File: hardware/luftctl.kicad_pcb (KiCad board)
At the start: 2 copper layers, 84 x 53.5 mm, 40 parts, among them J1 USB_C_Receptacle_USB2.0, J2 UART, J3 I2C, J4 PWM Fan, J5 PWM Fan, SW1 Reset, U1 LMR62014XMF, U2 MIC5504-3.3YM5, U3 USBLC6-4SC6, U4 ESP32-C3-WROOM-02

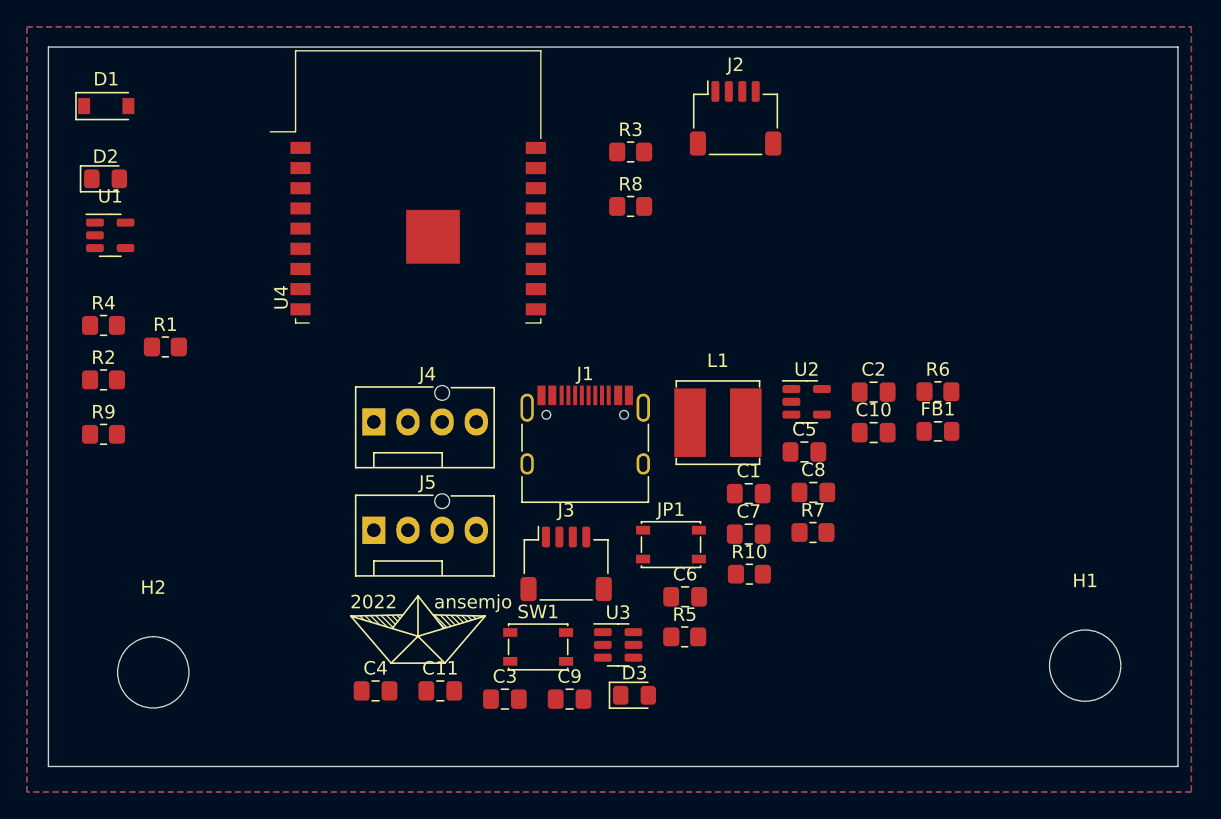
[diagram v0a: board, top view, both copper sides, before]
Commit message: finished pcb layout
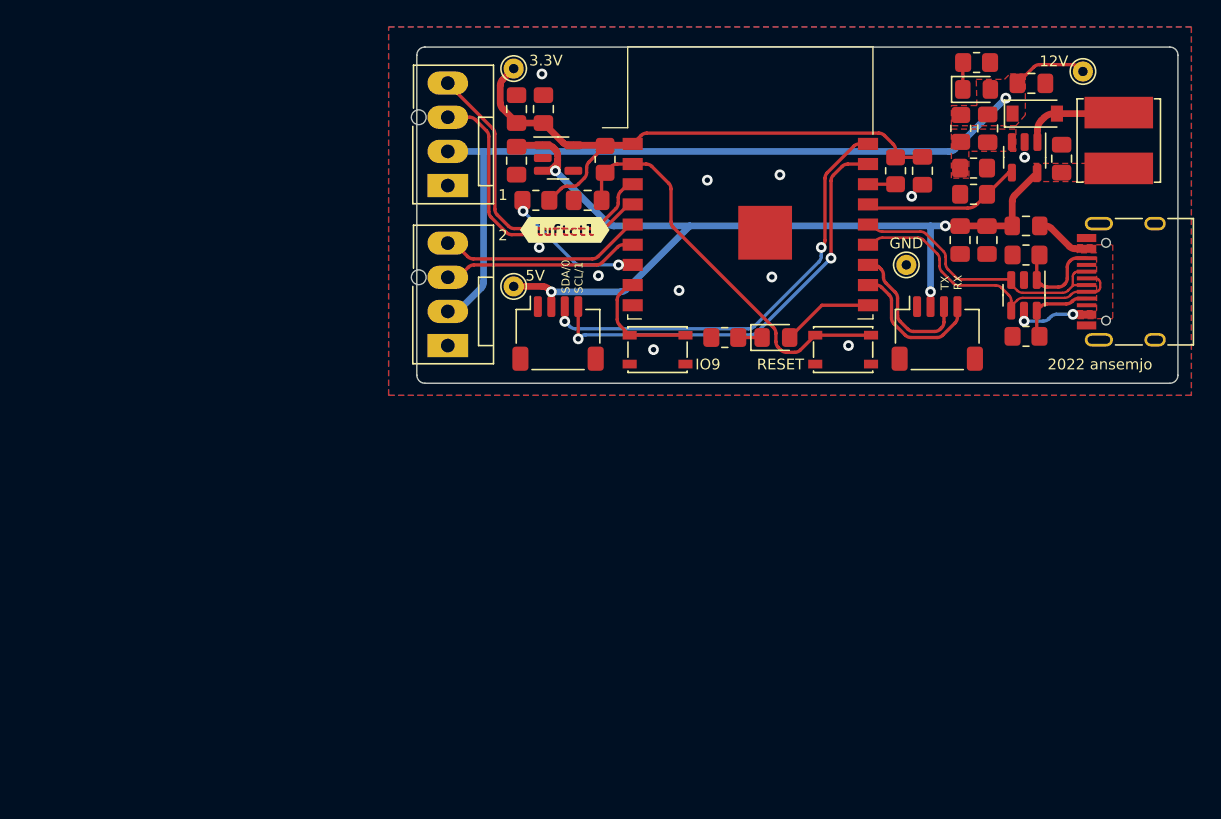
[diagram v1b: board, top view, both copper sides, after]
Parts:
- removed A1: 2022, ansemjo:ahoi
- removed C2: DNP, Capacitor_SMD:C_0805_2012Metric_Pad1.18x1.45mm_HandSolder
- removed H1, H2: MountingHole, MountingHole:MountingHole_5.3mm_M5
- added TP1: Test, TestPoint:TestPoint_THTPad_D1.5mm_Drill0.7mm, F.Cu at (175.1, 51.8)
- added TP2: Test, TestPoint:TestPoint_THTPad_D1.5mm_Drill0.7mm, F.Cu at (132.8, 67.8)
- added TP3: Test, TestPoint:TestPoint_THTPad_D1.5mm_Drill0.7mm, F.Cu at (132.8, 51.6)
- added TP4: Test, TestPoint:TestPoint_THTPad_D1.5mm_Drill0.7mm, F.Cu at (162.0, 66.2)
- added kibuzzard-61E47F36: G***, kibuzzard-61E47F36, F.Cu at (136.6, 63.6)
- moved D1 69.1 mm to (171.6, 55.0)
- moved R4 68.6 mm to (170.9, 71.5), turned to 180 degrees
- moved U1 68.2 mm to (170.8, 58.2), turned to -90 degrees
- moved R2 66.6 mm to (167.0, 59.0)
- moved R1 61.3 mm to (166.1, 56.0), turned to -90 degrees
- moved D3 51.7 mm to (167.2, 53.1)
- moved D2 51.2 mm to (152.3, 71.6)
- moved R9 46.8 mm to (148.5, 71.6), turned to 180 degrees
- moved C4 44.5 mm to (133.0, 54.6), turned to 90 degrees
- moved C11 43.9 mm to (135.0, 54.6), turned to -90 degrees
- moved J1 43.2 mm to (179.4, 67.5), turned to 90 degrees
- moved R10 41.6 mm to (167.2, 51.1)
- moved C6 41.5 mm to (168.1, 56.0), turned to -90 degrees
- moved C3 40.0 mm to (133.0, 58.5), turned to 90 degrees
- moved U3 39.8 mm to (170.8, 68.5), turned to -90 degrees
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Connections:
- FB1 pad 1: Net-(FB1-Pad1) -> VBUS
- J1 pad A4: Net-(FB1-Pad1) -> VBUS
- J1 pad A5: Net-(J1-PadA5) -> CC1
- J1 pad A9: Net-(FB1-Pad1) -> VBUS
- J1 pad B4: Net-(FB1-Pad1) -> VBUS
- J1 pad B5: Net-(J1-PadB5) -> CC2
- J1 pad B9: Net-(FB1-Pad1) -> VBUS
- J1 pad S1: Earth -> GND
- J4 pad 3: M1_Tacho -> FAN1_Tacho
- J4 pad 4: M1_PWM -> FAN1_PWM
- J5 pad 3: M2_Tacho -> FAN2_Tacho
- J5 pad 4: M2_PWM -> FAN2_PWM
- R4 pad 1: Net-(J1-PadA5) -> CC1
- R5 pad 2: Net-(J1-PadB5) -> CC2
- U3 pad 1: USB- -> CC2
- U3 pad 4: unconnected-(U3-Pad4) -> USB-
- U3 pad 5: +3V3 -> VBUS
- U3 pad 6: unconnected-(U3-Pad6) -> CC1
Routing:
- net +5V: track 0.00 -> 69.0 mm, vias 0 -> 4
- net +12V: track 0.00 -> 62.1 mm, vias 0 -> 1
- net +3V3: track 0.00 -> 43.5 mm
- net SDA: track 0.00 -> 32.9 mm, vias 0 -> 2
- net SCL: track 0.00 -> 32.7 mm, vias 0 -> 2
- net EN: track 0.00 -> 30.7 mm
- net FAN1_PWM: track 0.00 -> 23.5 mm
- net USB-: track 0.00 -> 23.0 mm
- net FAN1_Tacho: track 0.00 -> 21.7 mm
- net USB+: track 0.00 -> 21.0 mm
- net FAN2_PWM: track 0.00 -> 15.2 mm
- net FAN2_Tacho: track 0.00 -> 14.6 mm
- net 12V_EN: track 0.00 -> 11.9 mm
- net RXD: track 0.00 -> 10.7 mm
- net GPIO8: track 0.00 -> 10.6 mm, vias 0 -> 2
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- added copper zone on F.Cu, net +12V
- added copper zone on F.Cu, net +5V
- added copper zone on F.Cu, net Net-(C6-Pad2)
- added copper zone on F.Cu, net VBUS
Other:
- board size 84 x 53.5 mm -> 56.6 x 25 mm
- board text added: "1"
- board text added: "12V"
- board text added: "2"
- board text added: "2022 ansemjo"
- board text added: "3.3V"
- board text added: "5V"
- board text added: "GND"
- board text added: "IO9"
- board text added: "RESET"
- board text added: "SDA/0 SCL/1"
- board text added: "TX RX"
